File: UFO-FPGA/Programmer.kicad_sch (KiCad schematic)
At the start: 41 parts, among them U2 FT2232HL, U3 ASDMB-12MHz, U5 93LC56CT-I/MS

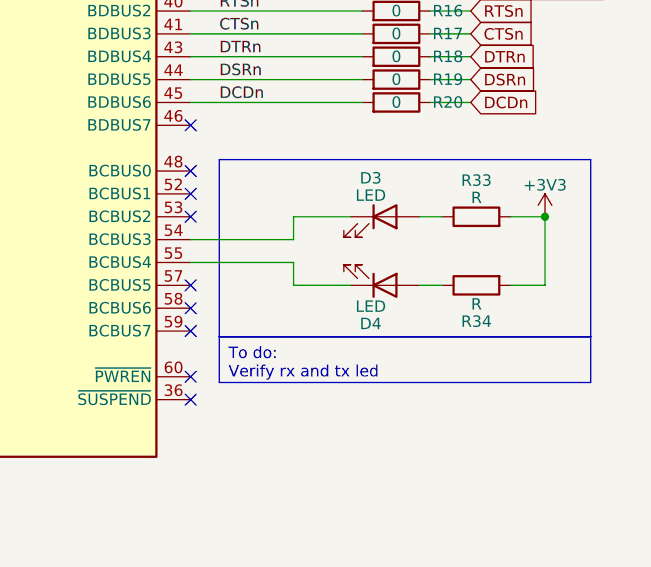
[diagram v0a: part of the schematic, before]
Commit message: edge cuts
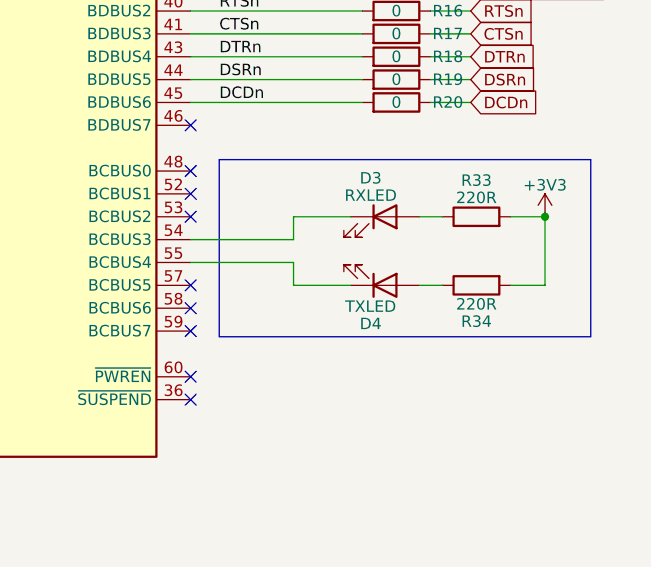
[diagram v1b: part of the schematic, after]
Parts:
- D3: value LED -> RXLED
- D4: value LED -> TXLED
- R33, R34: value R -> 220R
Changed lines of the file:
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@@
     (fill (type none))
-  )
-  (text_box "To do:\nVerify rx and tx led"
-    (at 287.655 168.275 0) (size 41.275 5.08)
-    (stroke (width 0) (type default))
-    (fill (type none))
-    (effects (font (size 1.27 1.27)) (justify left top))
   )
   (text "12MHz oscillator" (at 149.225 161.925 0)
@@
       (effects (font (size 1.27 1.27)))
     )
-    (property "Value" "R" (at 316.23 152.8351 90)
+    (property "Value" "220R" (at 316.23 152.8351 90)
       (effects (font (size 1.27 1.27)))
     )
@@
       (effects (font (size 1.27 1.27)))
     )
-    (property "Value" "LED" (at 304.4825 164.9189 0)
+    (property "Value" "TXLED" (at 304.4825 164.9189 0)
       (effects (font (size 1.27 1.27)))
     )
@@
       (effects (font (size 1.27 1.27)))
     )
-    (property "Value" "R" (at 316.23 164.6649 90)
+    (property "Value" "220R" (at 316.23 164.6649 90)
       (effects (font (size 1.27 1.27)))
     )
@@
       (effects (font (size 1.27 1.27)))
     )
-    (property "Value" "LED" (at 304.4825 152.5811 0)
-      (effects (font (size 1.27 1.27)))
-    )
+    (property "Value" "RXLED" (at 304.4825 152.5811 0)
+      (effects (font (size 1.27 1.27)))
+    )
